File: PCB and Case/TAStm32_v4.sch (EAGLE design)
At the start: 55 parts, among them CN1 330pF, CN2 330pF, CN3 330pF, CN4 330pF, IC1 74LVC3G17DP, IC2 74LVC3G17DP, IC3 74AXP4T245, IC4 74AXP4T245, J1 ZX62D-B-5PA8, J10 RJSSE538002, J11 RJSSE538002, J12 SOICBITE, J13 CONSOLE_RESET, J2 UE27-AC54-100, J3 TSM-105-02-L-SHJ, J4 CONSOLE_RESET, J5 OLED128X64, J6 SAMTEC-TSM-116-01-X-SVJ, J7 SAMTEC-TSM-116-01-X-SVJ, U1 STM32F446RET6, U2 3.3V REG, Y1 8MHz

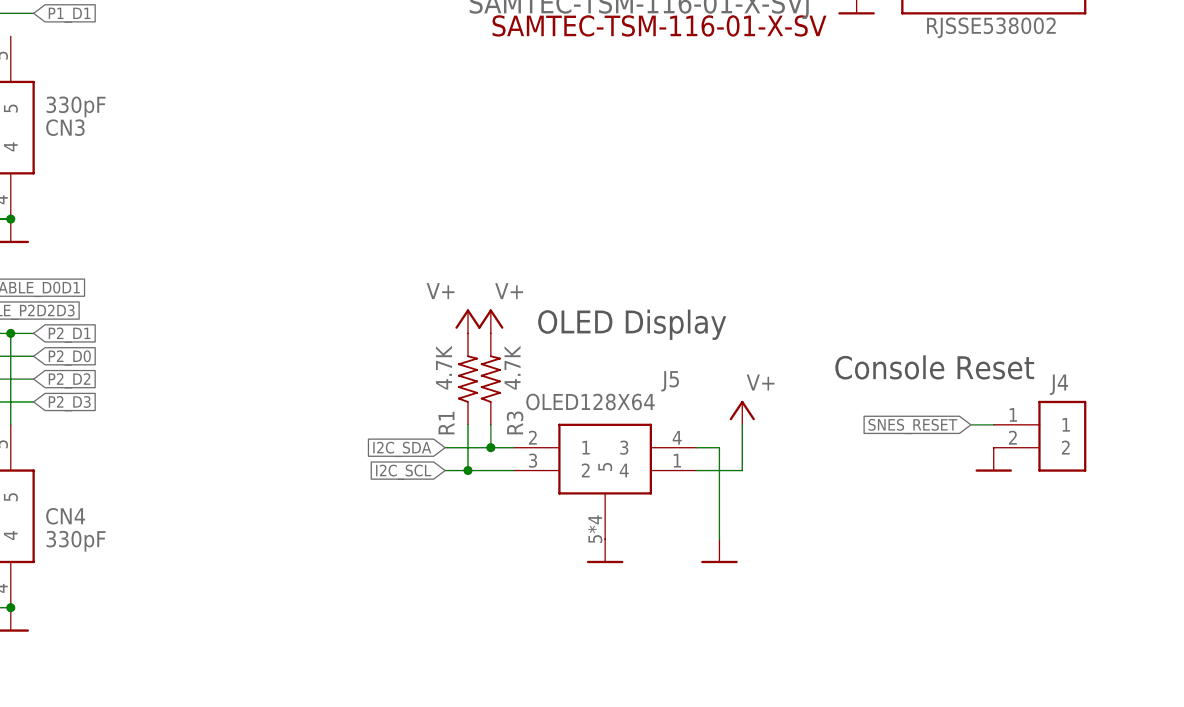
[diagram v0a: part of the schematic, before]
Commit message: 3D parts
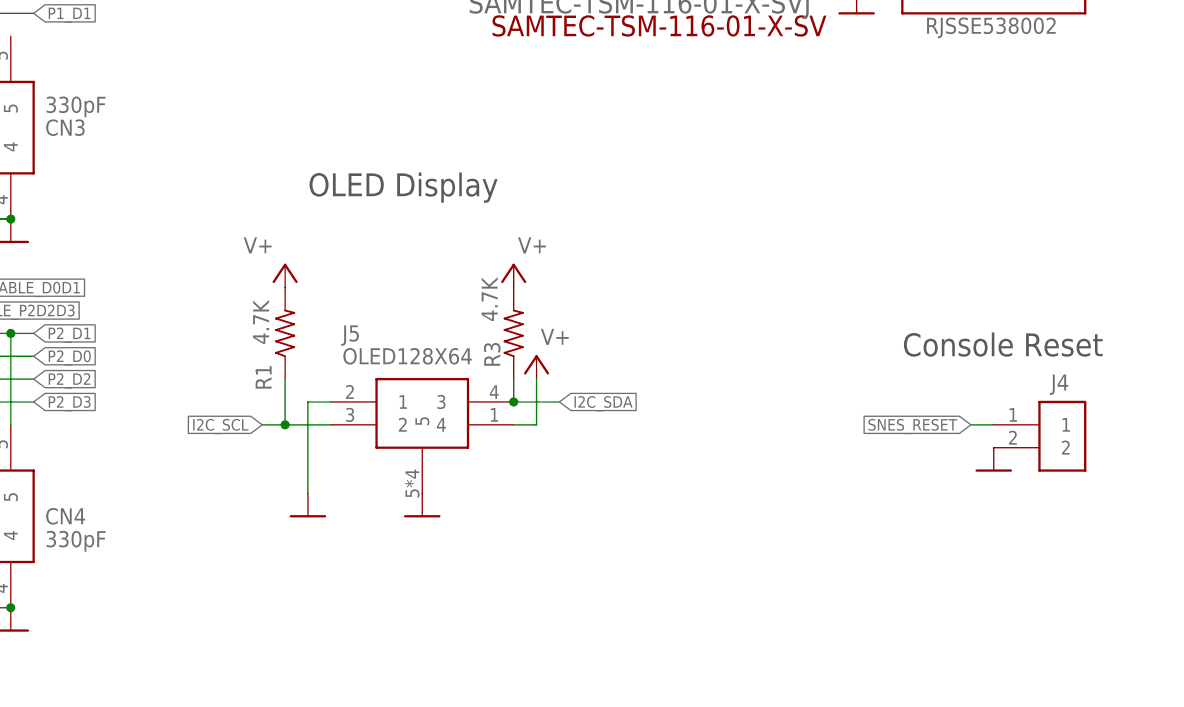
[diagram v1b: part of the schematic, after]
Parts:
- C1, C10, C11, C12, C13, C14, C15, C16, C17, C2, C3, C4, C5, C6, C7, C8, C9: device rcl:C-EUC0603K -> TAStm32_v4:C-EUC0603K
- CN1, CN2, CN3, CN4: device SamacSys_Parts:CA0612KRX7R7BB104 -> TAStm32_v4:CA0612KRX7R7BB104
- IC1, IC2: device SamacSys_Parts:74HCT3G07DP-Q100H -> TAStm32_v4:74HCT3G07DP-Q100H
- IC3, IC4: device SamacSys_Parts:74AVCH4T245PW,118 -> TAStm32_v4:74AVCH4T245PW,118
- J1: device ZX62D-B-5PA8:ZX62D-B-5PA8 -> TAStm32_v4:ZX62D-B-5PA8
- J12: device SOICbite_Eagle:SOICBITE -> TAStm32_v4:SOICBITE
- J2: device SamacSys_Parts:UE27-AC54-100 -> TAStm32_v4:UE27-AC54-100
- J3: device TSM-105-02-L-SH:TSM-105-02-L-SHJ -> TAStm32_v4:TSM-105-02-L-SHJ
- J6, J7: device SAMTEC-TSM-116-01-X-SV:SAMTEC-TSM-116-01-X-SVJ -> TAStm32_v4:SAMTEC-TSM-116-01-X-SVJ
- R1, R2, R3: device rcl:R-US_R0805 -> TAStm32_v4:R-US_R0805
- RN1, RN2, RN3, RN4, RN5, RN7: device resistor-net:CTS742C083 -> TAStm32_v4:CTS742C083
- U1: device STM32F446RET6:STM32F446RET7 -> TAStm32_v4:STM32F446RET7
- U2: device linear:MC33269ST-3.3T3 -> TAStm32_v4:MC33269ST-3.3T3
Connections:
- net GND: now also J5.1; no longer J5.3
- net I2C_SDA: now also J5.3; no longer J5.1
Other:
- moved on the sheet: J5, R1, R3
